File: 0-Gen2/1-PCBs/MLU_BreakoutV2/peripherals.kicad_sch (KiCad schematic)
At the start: 88 parts, among them J10 Conn_02x03_Odd_Even, J11 430450422, J12 PixHawk PM02, J14 Conn_01x02_Socket, J17 430450422, J18 430450422, J19 430450422, J2 430450422, J20 430450228, J21 430450228, J22 430450228, J23 430450228, J25 430450228, J26 430450821, J28 Conn_01x04_Socket, J3 Conn_01x03_Pin, J31 Conn_01x02_Socket, J4 430450422, J5 430451027, J8 Conn_02x22_Odd_Even, J9 J1B1211CCD

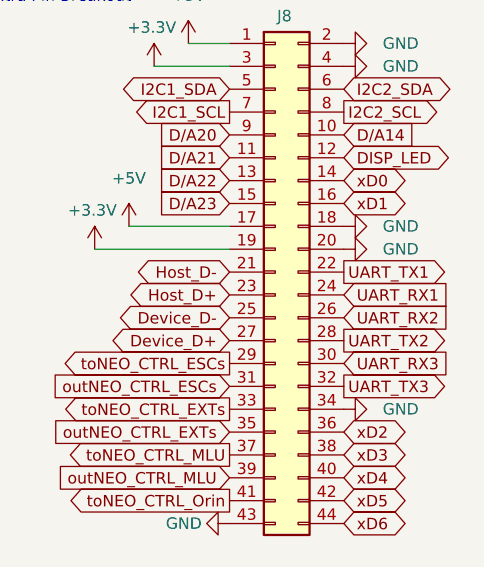
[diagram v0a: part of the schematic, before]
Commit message: [add] beginning routing
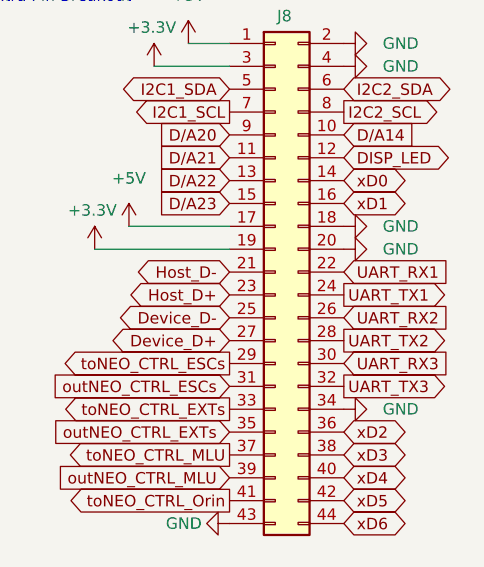
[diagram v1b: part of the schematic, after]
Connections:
- net UART_RX1: now also J8.22 (Pin_22); no longer J8.24 (Pin_24)
- net UART_TX1: now also J8.24 (Pin_24); no longer J8.22 (Pin_22)
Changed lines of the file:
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@@
 	(global_label "UART_RX1"
 		(shape input)
-		(at 239.776 128.778 0)
-		(fields_autoplaced yes)
-		(effects
-			(font
-				(size 1.27 1.27)
-			)
-			(justify left)
-		)
-		(property "Intersheetrefs" "${INTERSHEET_REFS}"
-			(at 252.0745 128.778 0)
+		(at 239.776 126.238 0)
+		(fields_autoplaced yes)
+		(effects
+			(font
+				(size 1.27 1.27)
+			)
+			(justify left)
+		)
+		(property "Intersheetrefs" "${INTERSHEET_REFS}"
+			(at 252.0745 126.238 0)
 			(effects
 				(font
@@
 	(global_label "UART_TX1"
 		(shape output)
-		(at 239.776 126.238 0)
-		(fields_autoplaced yes)
-		(effects
-			(font
-				(size 1.27 1.27)
-			)
-			(justify left)
-		)
-		(property "Intersheetrefs" "${INTERSHEET_REFS}"
-			(at 251.7721 126.238 0)
-			(effects
-				(font
+		(at 239.776 128.778 0)
+		(fields_autoplaced yes)
+		(effects
+			(font
+				(size 1.27 1.27)
+			)
+			(justify left)
+		)
+		(property "Intersheetrefs" "${INTERSHEET_REFS}"
+			(at 251.7721 128.778 0)
+			(effects
+				(font

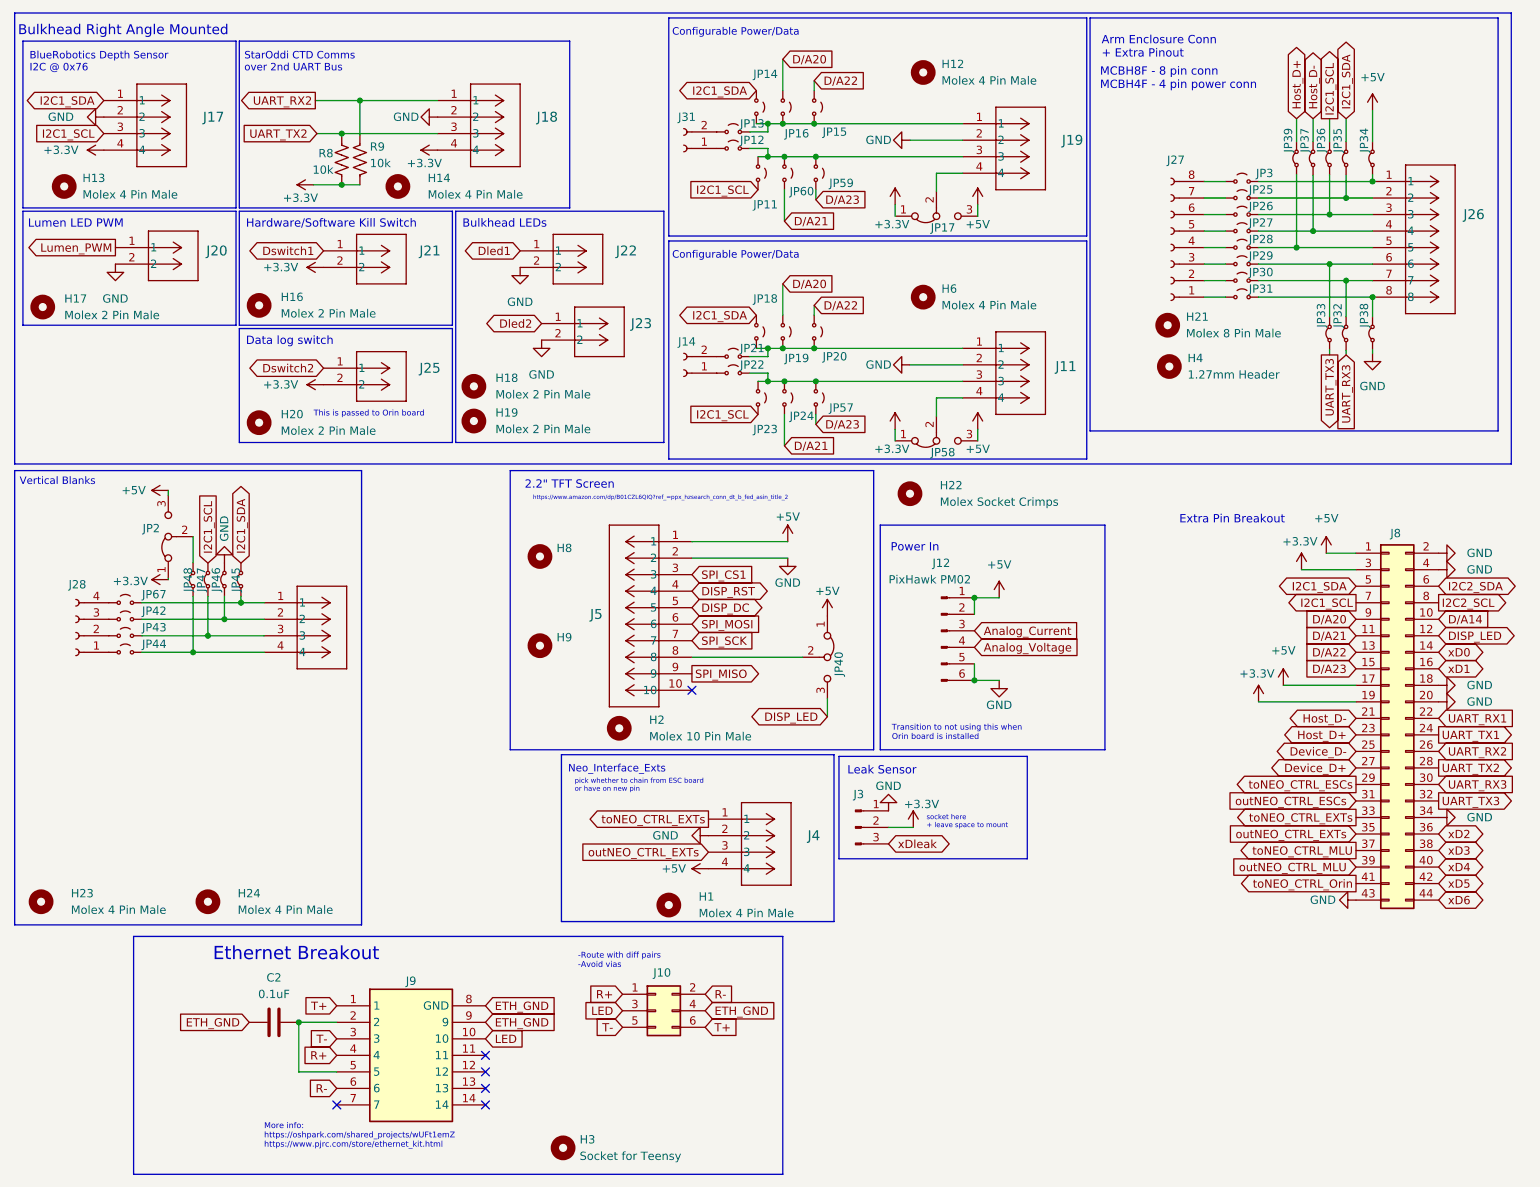
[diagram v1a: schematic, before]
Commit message: before restructure
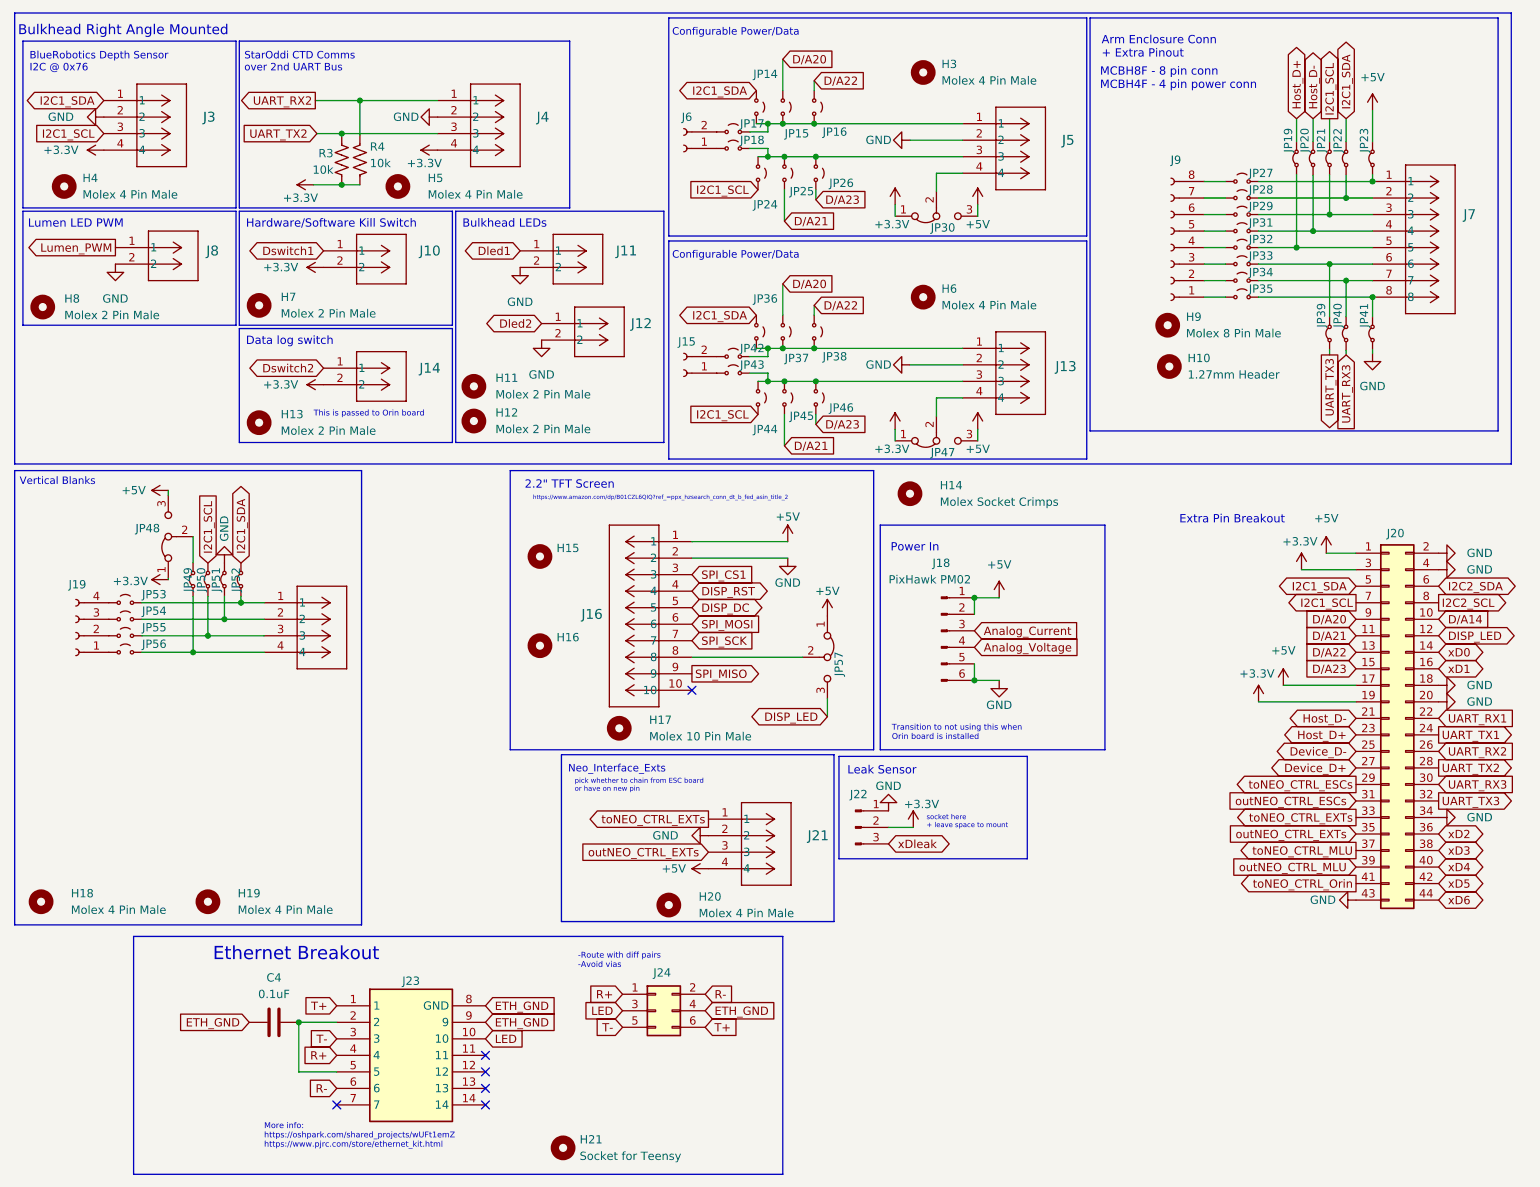
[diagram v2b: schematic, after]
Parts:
- renumbered C2 to C4, H4 to H10, H18 to H11, H19 to H12, H20 to H13, H22 to H14, H8 to H15, H9 to H16, H2 to H17, H23 to H18, H24 to H19, H1 to H20, H3 to H21, H12 to H3, H13 to H4, H14 to H5, H16 to H7, H17 to H8, H21 to H9, J21 to J10, J22 to J11, J23 to J12, J11 to J13, J25 to J14, J14 to J15, J5 to J16, J2 to J17, J12 to J18, J28 to J19, J8 to J20, J4 to J21, J3 to J22, J9 to J23, J10 to J24, J17 to J3, J18 to J4, J19 to J5, J31 to J6, J26 to J7, J20 to J8, J27 to J9, JP16 to JP15, JP15 to JP16, JP13 to JP17, JP12 to JP18, JP39 to JP19, JP37 to JP20, JP36 to JP21, JP35 to JP22, JP34 to JP23, JP11 to JP24, JP60 to JP25, JP59 to JP26, JP3 to JP27, JP25 to JP28, JP26 to JP29, JP17 to JP30, JP27 to JP31, JP28 to JP32, JP29 to JP33, JP30 to JP34, JP31 to JP35, JP18 to JP36, JP19 to JP37, JP20 to JP38, JP33 to JP39, JP32 to JP40, JP38 to JP41, JP21 to JP42, JP22 to JP43, JP23 to JP44, JP24 to JP45, JP57 to JP46, JP58 to JP47, JP2 to JP48, JP48 to JP49, JP47 to JP50, JP46 to JP51, JP45 to JP52, JP67 to JP53, JP42 to JP54, JP43 to JP55, JP44 to JP56, JP40 to JP57, R8 to R3, R9 to R4
